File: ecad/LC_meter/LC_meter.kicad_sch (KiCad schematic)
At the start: 21 parts, among them J2 Display Connector, J3 12V Power, U5 LTC1044, U6 LM7805_TO220

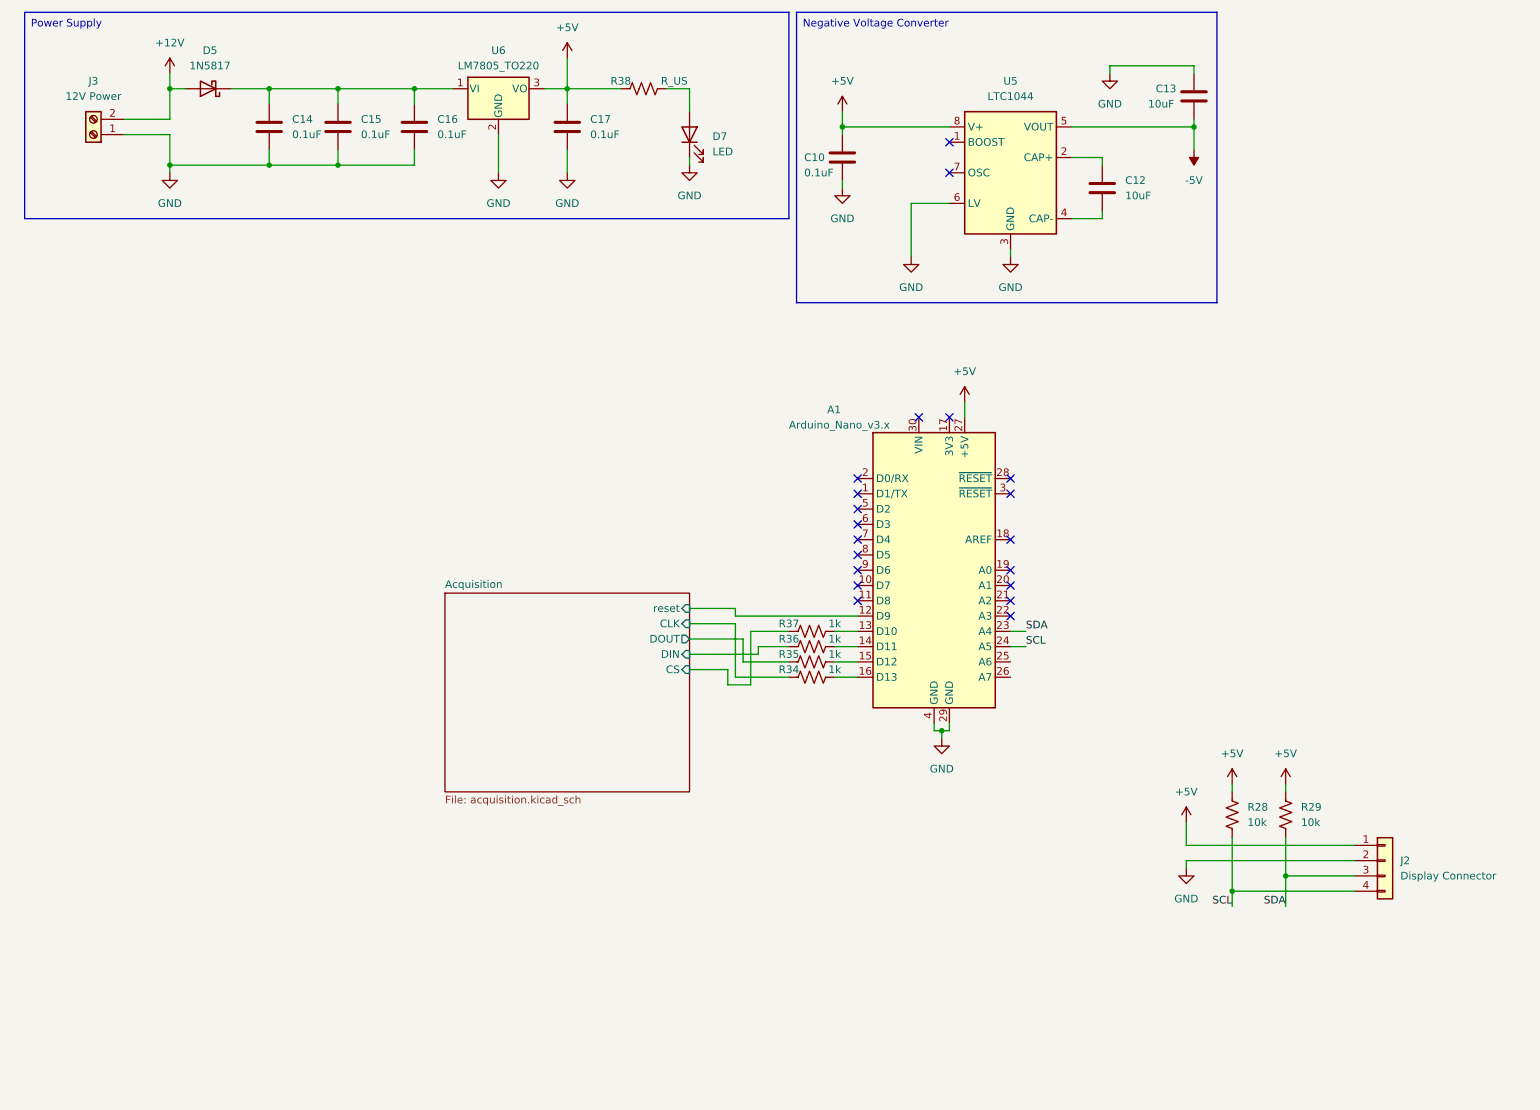
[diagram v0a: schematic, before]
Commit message: ok range calcs and schematic
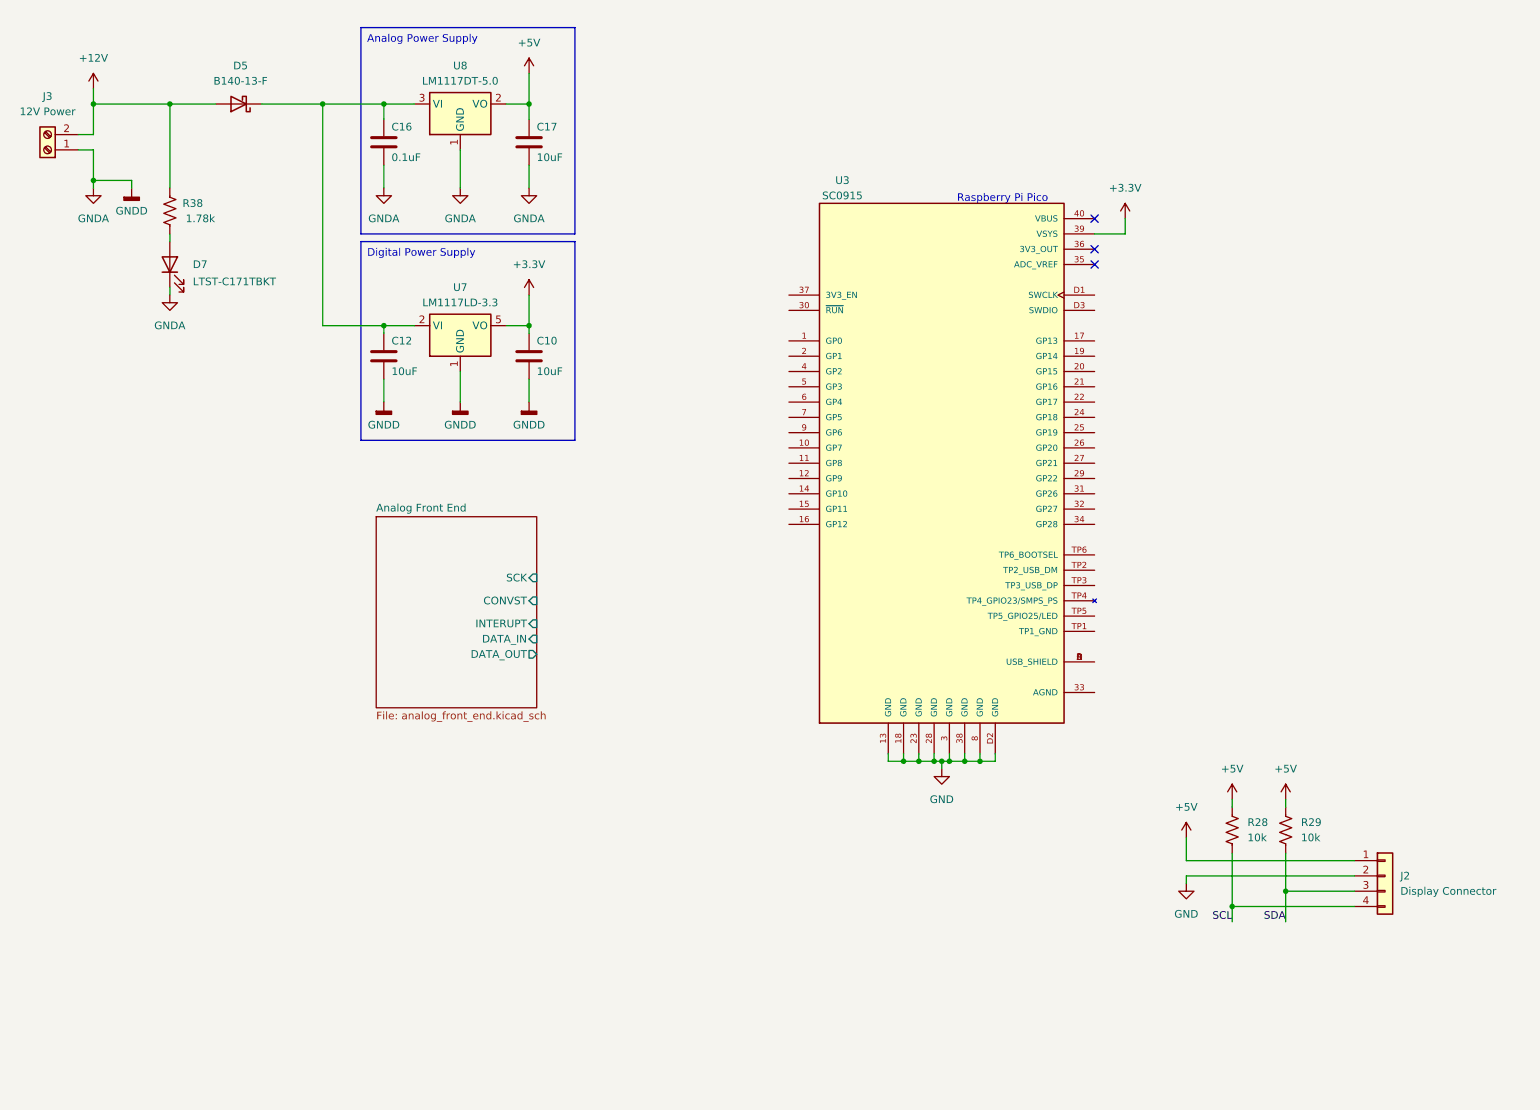
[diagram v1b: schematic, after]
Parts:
- removed A1: Arduino_Nano_v3.x, Module:Arduino_Nano, symbol MCU_Module:Arduino_Nano_v3.x
- removed C13: 10uF, symbol Device:C
- removed C14, C15: 0.1uF, symbol Device:C
- removed R34, R35, R36, R37: 1k, symbol Device:R_US
- removed U5: LTC1044, symbol Regulator_SwitchedCapacitor:LTC1044
- removed U6: LM7805_TO220, Package_TO_SOT_THT:TO-220-3_Vertical, symbol Regulator_Linear:LM7805_TO220
- added U3: SC0915, SC0915:MODULE_SC0915, symbol LCR_parts:SC0915
- added U7: LM1117LD-3.3, Package_SON:WSON-8-1EP_4x4mm_P0.8mm_EP2.2x3mm, symbol Regulator_Linear:LM1117LD-3.3
- added U8: LM1117DT-5.0, Package_TO_SOT_SMD:TO-252-3_TabPin2, symbol Regulator_Linear:LM1117DT-5.0
- C10, C17: value 0.1uF -> 10uF
- D5: value 1N5817 -> B140-13-F
- D7: value LED -> LTST-C171TBKT
- R38: value R_US -> 1.78k
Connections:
- net +12V: now also R38.2
- net +5V: now also U8.2 (VO); no longer C10.1, R38.1
- net GND: now also U3.13 (GND), U3.18 (GND), U3.23 (GND), U3.28 (GND), U3.3 (GND), U3.38 (GND), U3.8 (GND), U3.D2 (GND); no longer C10.2, C16.2, C17.2, D7.1 (K), J3.1 (Pin_1)
- net at D7.2 (A): now also R38.1; no longer R38.2
- net at C16.1, D5.1 (K): now also C12.1, U7.2 (VI), U7.3 (VI), U7.4 (VI), U8.3 (VI)
- net GNDA: now reaches C12.2
- net GNDA: now also C10.2, C16.2, C17.2, D7.1 (K), J3.1 (Pin_1), U7.1 (GND), U8.1 (GND)
- new net: U3.A (USB_SHIELD), U3.B (USB_SHIELD), U3.C (USB_SHIELD), U3.D (USB_SHIELD)
- new net +3.3V: C10.1, U3.39 (VSYS), U7.5 (VO), U7.6 (VO), U7.7 (VO), U7.9 (VO)
- no-connect marks 20 -> 3
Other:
- removed sheet Acquisition
- added sheet Analog Front End (analog_front_end.kicad_sch)
- note added: "Raspberry Pi Pico"
- moved on the sheet: C16, C17, D5, D7, J2, J3, R28, R29, R38

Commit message: crashed
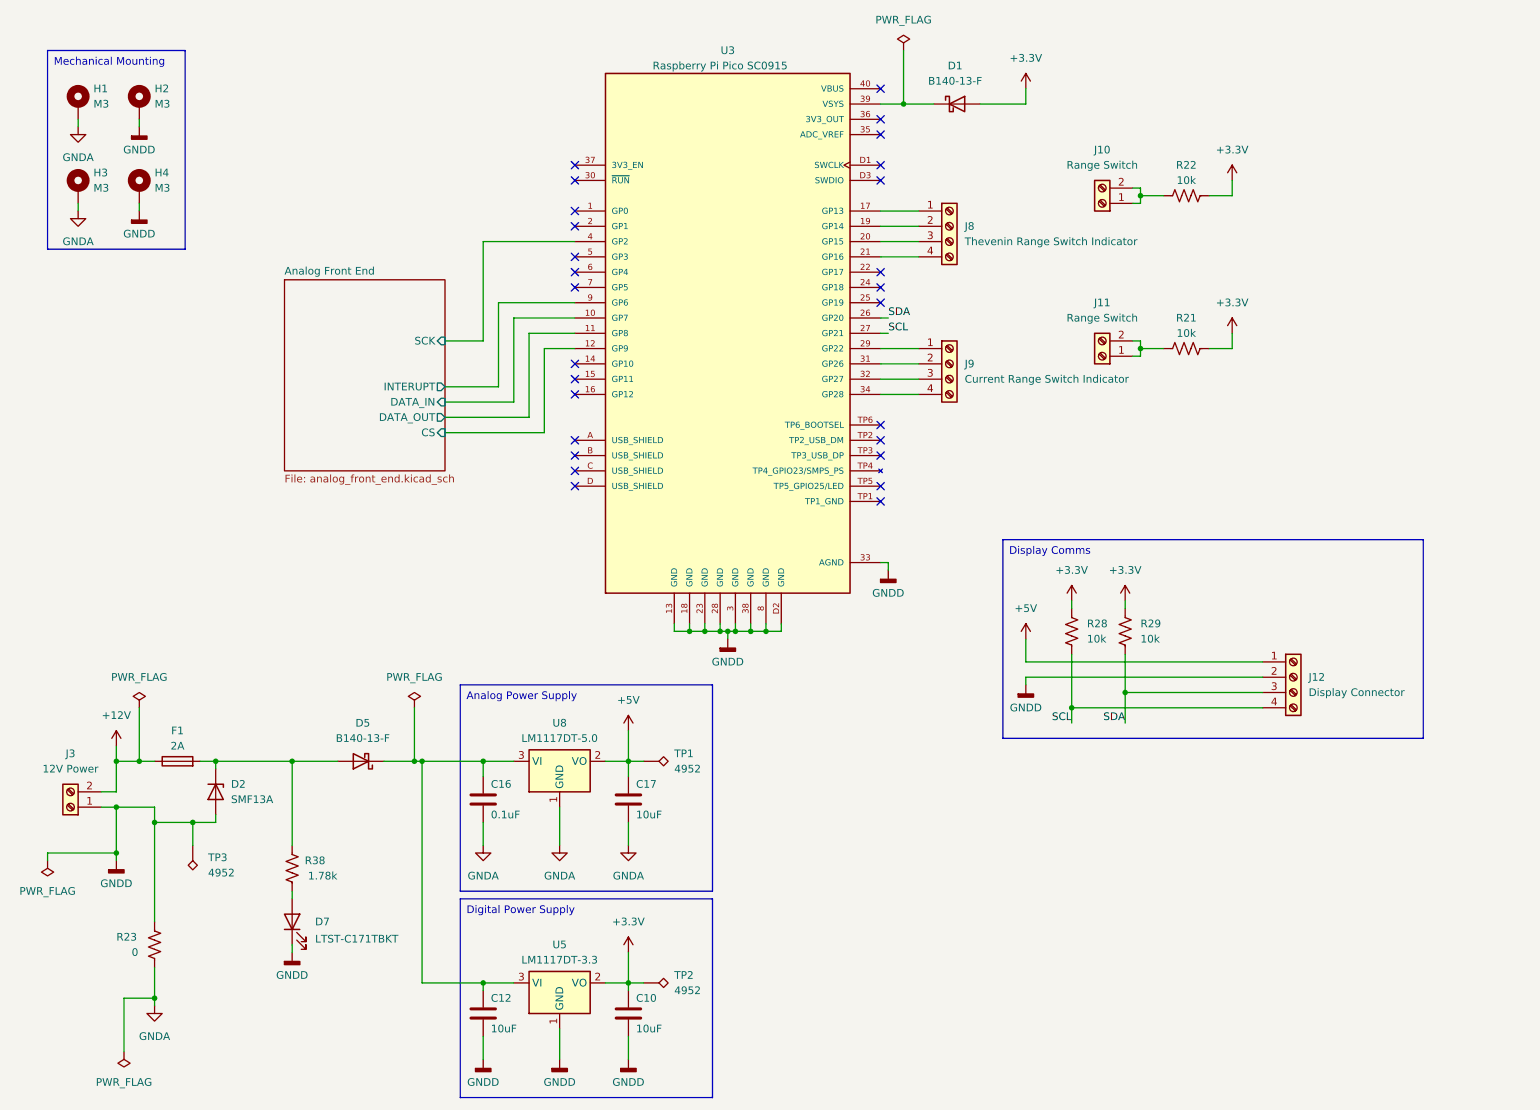
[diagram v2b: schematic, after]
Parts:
- removed J2: Display Connector, symbol Connector_Generic:Conn_01x04
- removed U7: LM1117LD-3.3, Package_SON:WSON-8-1EP_4x4mm_P0.8mm_EP2.2x3mm, symbol Regulator_Linear:LM1117LD-3.3
- added D1: B140-13-F, Diode_SMD:D_SMA, symbol Diode:1N5817
- added D2: SMF13A, Diode_SMD:D_SOD-123F, symbol Device:D_Zener
- added F1: 2A, Fuse:Fuse_0805_2012Metric, symbol Device:Fuse
- added H1, H2, H3, H4: M3, MountingHole:MountingHole_3.2mm_M3_Pad_Via, symbol Mechanical:MountingHole_Pad
- added J10, J11: Range Switch, TerminalBlock_Phoenix:TerminalBlock_Phoenix_MPT-0,5-2-2.54_1x02_P2.54mm_Horizontal, symbol Connector:Screw_Terminal_01x02
- added J12: Display Connector, TerminalBlock_Phoenix:TerminalBlock_Phoenix_MPT-0,5-4-2.54_1x04_P2.54mm_Horizontal, symbol Connector:Screw_Terminal_01x04
- added J8: Thevenin Range Switch Indicator, TerminalBlock_Phoenix:TerminalBlock_Phoenix_MPT-0,5-4-2.54_1x04_P2.54mm_Horizontal, symbol Connector:Screw_Terminal_01x04
- added J9: Current Range Switch Indicator, TerminalBlock_Phoenix:TerminalBlock_Phoenix_MPT-0,5-4-2.54_1x04_P2.54mm_Horizontal, symbol Connector:Screw_Terminal_01x04
- added R21, R22: 10k, Resistor_SMD:R_0805_2012Metric, symbol Device:R_US
- added R23: 0, Resistor_SMD:R_0805_2012Metric, symbol Device:R_US
- added TP1, TP2, TP3: 4952, Connector_Pin:Pin_D1.2mm_L10.2mm_W2.9mm_FlatFork, symbol Connector:TestPoint_Alt
- added U5: LM1117DT-3.3, Package_TO_SOT_SMD:TO-252-3_TabPin2, symbol Regulator_Linear:LM1117DT-3.3
- C10, C12, C16, C17: footprint (none) -> Capacitor_SMD:C_0805_2012Metric
- D5: footprint Diode_THT:D_DO-41_SOD81_P10.16mm_Horizontal -> Diode_SMD:D_SMA
- D7: footprint (none) -> LED_SMD:LED_0805_2012Metric
- J3: footprint (none) -> TerminalBlock_Phoenix:TerminalBlock_Phoenix_MPT-0,5-2-2.54_1x02_P2.54mm_Horizontal
- R28, R29, R38: footprint (none) -> Resistor_SMD:R_0805_2012Metric
- U3: value SC0915 -> Raspberry Pi Pico SC0915; footprint SC0915:MODULE_SC0915 -> LC_meter:MODULE_SC0915
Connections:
- net GND is gone; now on net GNDD: U3.13 (GND), U3.18 (GND), U3.23 (GND), U3.28 (GND), U3.3 (GND), U3.38 (GND), U3.8 (GND), U3.D2 (GND)
- net +12V: now also F1.1; no longer D5.2 (A), R38.2
- net +3.3V: now also R28.1, R29.1, D1.2 (A), R21.1, R22.1, TP2.1, U5.2 (VO); no longer U3.39 (VSYS)
- net +5V: now also J12.1 (Pin_1), TP1.1; no longer R28.1, R29.1
- net Analog Front End/DATA_IN: now also U3.10 (GP7)
- net Analog Front End/DATA_OUT: now also U3.11 (GP8)
- net Analog Front End/INTERUPT: now also U3.9 (GP6)
- net Analog Front End/SCK: now also U3.4 (GP2)
- net GNDA: now also H1.1, H3.1, R23.2; no longer C10.2, C12.2, D7.1 (K), J3.1 (Pin_1)
- net SCL: now also U3.27 (GP21), J12.4 (Pin_4)
- net SDA: now also U3.26 (GP20), J12.3 (Pin_3)
- net at C12.1, C16.1, D5.1 (K)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: now also U5.3 (VI)
- net Analog Front End/CS: now reaches U3.12 (GP9)
- net at U3.17 (GP13): now also J8.1 (Pin_1)
- net at U3.19 (GP14): now also J8.2 (Pin_2)
- net at U3.20 (GP15): now also J8.3 (Pin_3)
- net at U3.21 (GP16): now also J8.4 (Pin_4)
- net at U3.29 (GP22): now also J9.1 (Pin_1)
- net at U3.31 (GP26): now also J9.2 (Pin_2)
- net at U3.32 (GP27): now also J9.3 (Pin_3)
- net GNDD: now reaches U3.33 (AGND)
- net GNDD: now also C10.2, C12.2, D7.1 (K), J3.1 (Pin_1), D2.2 (A), H2.1, H4.1, J12.2 (Pin_2), R23.1, TP3.1, U5.1 (GND)
- net at U3.34 (GP28): now also J9.4 (Pin_4)
- new net: J11.1 (Pin_1), J11.2 (Pin_2), R21.2
- new net: D1.1 (K), U3.39 (VSYS)
- new net: D2.1 (K), D5.2 (A), F1.2, R38.2
- new net: J10.1 (Pin_1), J10.2 (Pin_2), R22.2
- now unconnected: U3.A (USB_SHIELD), U3.B (USB_SHIELD), U3.C (USB_SHIELD), U3.D (USB_SHIELD)
- no-connect marks 3 -> 27
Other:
- sheet Analog Front End ports: added CS; removed CONVST
- note removed: "Raspberry Pi Pico"
- moved on the sheet: C10, C12, C16, C17, D5, D7, J3, R28, R29, R38, U8
